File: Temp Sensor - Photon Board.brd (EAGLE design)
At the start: 43.8 x 52.7 mm, 16 parts

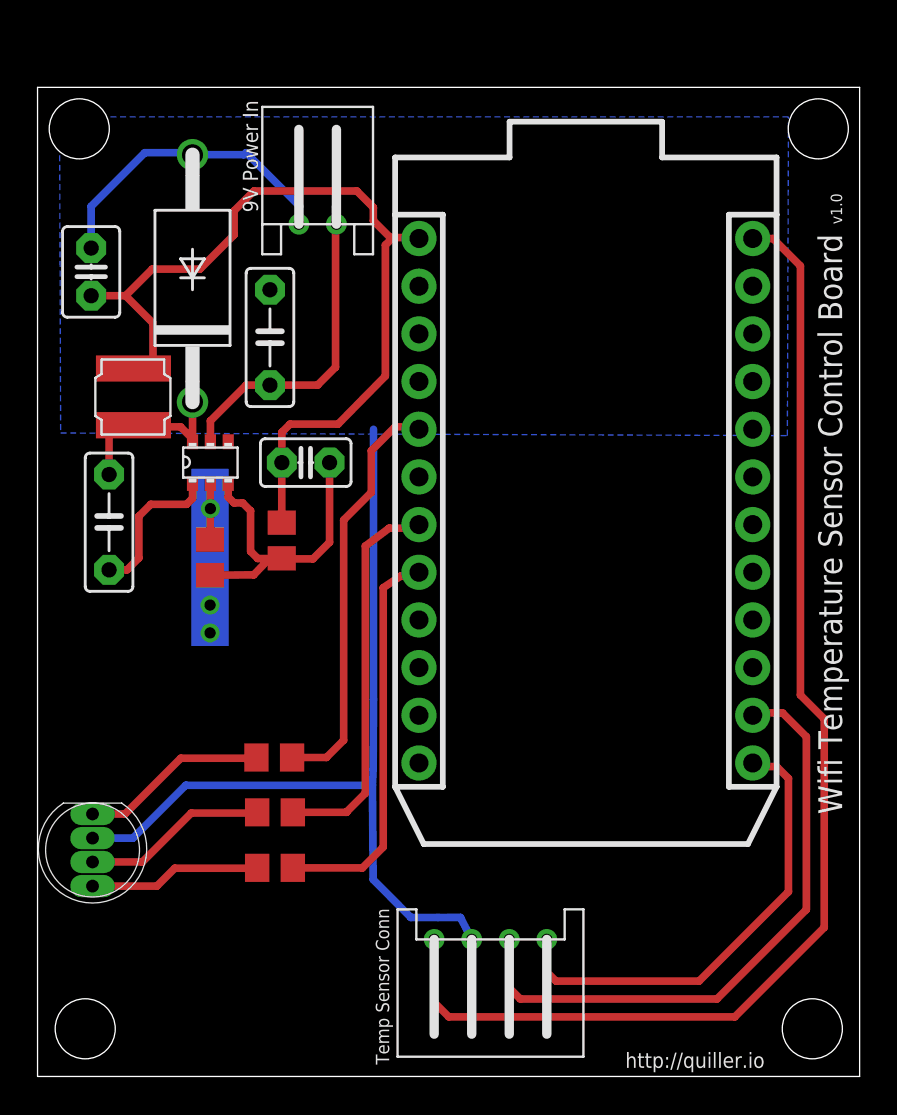
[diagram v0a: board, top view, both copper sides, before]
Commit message: Added Temp Sensor gerber files.  General cleanup or bck files
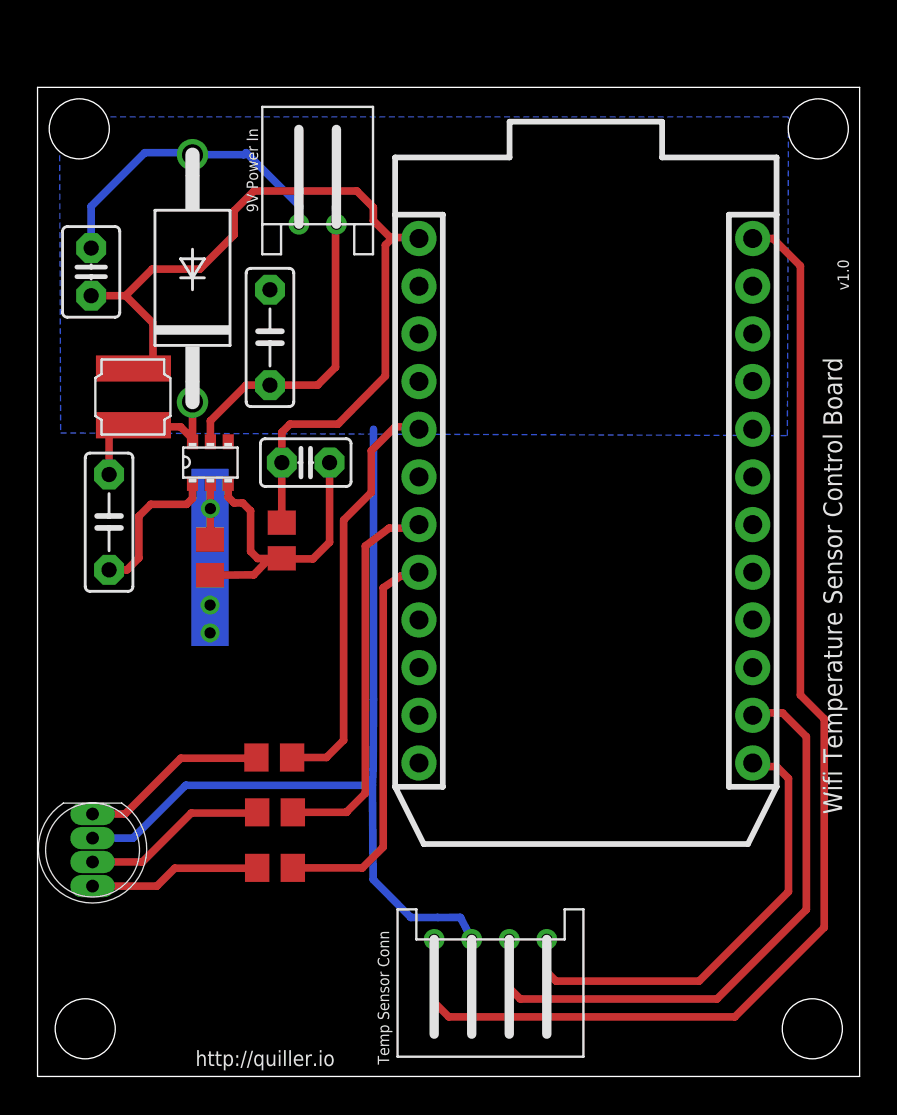
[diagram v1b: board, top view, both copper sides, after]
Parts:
- U$15: value 50 -> 100
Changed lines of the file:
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@@
 <layer number="21" name="tPlace" color="7" fill="1" visible="yes" active="yes"/>
 <layer number="22" name="bPlace" color="7" fill="1" visible="yes" active="yes"/>
-<layer number="23" name="tOrigins" color="15" fill="1" visible="yes" active="yes"/>
-<layer number="24" name="bOrigins" color="15" fill="1" visible="yes" active="yes"/>
+<layer number="23" name="tOrigins" color="15" fill="1" visible="no" active="yes"/>
+<layer number="24" name="bOrigins" color="15" fill="1" visible="no" active="yes"/>
 <layer number="25" name="tNames" color="7" fill="1" visible="yes" active="yes"/>
 <layer number="26" name="bNames" color="7" fill="1" visible="yes" active="yes"/>
@@
 <text x="60.325" y="99.3775" size="0.508" layer="27" align="center">9V</text>
 <text x="58.42" y="99.3775" size="0.508" layer="27" rot="R180" align="center">GND</text>
-<text x="56.1975" y="93.345" size="0.8128" layer="25" rot="R90">9V Power In</text>
-<text x="63.1825" y="47.9425" size="0.7112" layer="25" rot="R90">Temp Sensor Conn</text>
-<text x="87.3125" y="61.2775" size="1.27" layer="25" rot="R90">Wifi Temperature Sensor Control Board</text>
-<text x="87.3125" y="92.71" size="0.6096" layer="25" rot="R90">v1.0</text>
-<text x="83.185" y="48.5775" size="0.8128" layer="25" rot="R180">http://quiller.io</text>
+<text x="56.1975" y="93.345" size="0.6096" layer="25" rot="R90">9V Power In</text>
+<text x="63.1825" y="47.9425" size="0.6096" layer="25" rot="R90">Temp Sensor Conn</text>
+<text x="87.3125" y="61.2775" size="1" layer="25" rot="R90">Wifi Temperature Sensor Control Board</text>
+<text x="87.6725" y="89.19" size="0.6096" layer="25" rot="R90">v1.0</text>
+<text x="60.285" y="48.6775" size="0.8128" layer="25" rot="R180">http://quiller.io</text>
 <rectangle x1="52.64" y1="70.24" x2="54.64" y2="79.68" layer="16"/>
 <text x="53.3" y="74.82" size="0.3048" layer="27">680</text>
@@
 <element name="U$1" library="myhvac" package="JST_PH-2" value="" x="59.3725" y="92.71" rot="R180"/>
 <element name="D1" library="myhvac" package="LED-RGB-THR" value="LED-RGB-CC-THRU" x="47.38" y="59.37" rot="R90"/>
-<element name="U$15" library="myhvac" package="R0805" value="50" x="57.06" y="64.3" smashed="yes"/>
+<element name="U$15" library="myhvac" package="R0805" value="100" x="57.06" y="64.3" smashed="yes"/>
 <element name="U$16" library="myhvac" package="R0805" value="100" x="57.1" y="61.38" smashed="yes"/>
 <element name="U$17" library="myhvac" package="R0805" value="100" x="57.1" y="58.42" smashed="yes"/>
